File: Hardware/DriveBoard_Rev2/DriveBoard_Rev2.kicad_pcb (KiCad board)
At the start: 2 copper layers, 152.4 x 101.6 mm, 139 parts, among them J1 RJ45_LED_Shielded, Q1 Q_NMOS_DGS, Q2 Q_NMOS_DGS, Q3 Q_NMOS_DGS, Q4 Q_NMOS_DGS, Q5 Q_NMOS_DGS, Q6 Q_NMOS_DGS, Q7 Q_NMOS_DGS, Q8 Q_NMOS_DGS, Q9 Q_NMOS_DGS, SW1 SW_Push, SW10 SW_Push, SW11 SW_Push, SW12 SW_Push, SW13 SW_Push, SW14 SW_Push, SW15 SW_Push, SW16 SW_SPDT, SW2 SW_Push, SW3 SW_Push, SW4 SW_Push, SW5 SW_Push, SW6 SW_Push, SW7 SW_Push, SW8 SW_Push, SW9 SW_Push, U1 Teensy4.1_DEV-16771, U2 TSR_1-2450, U3 OKI, U4 74HC148, U5 74HC148, U6 74HC00, U7 TSR_1-2450

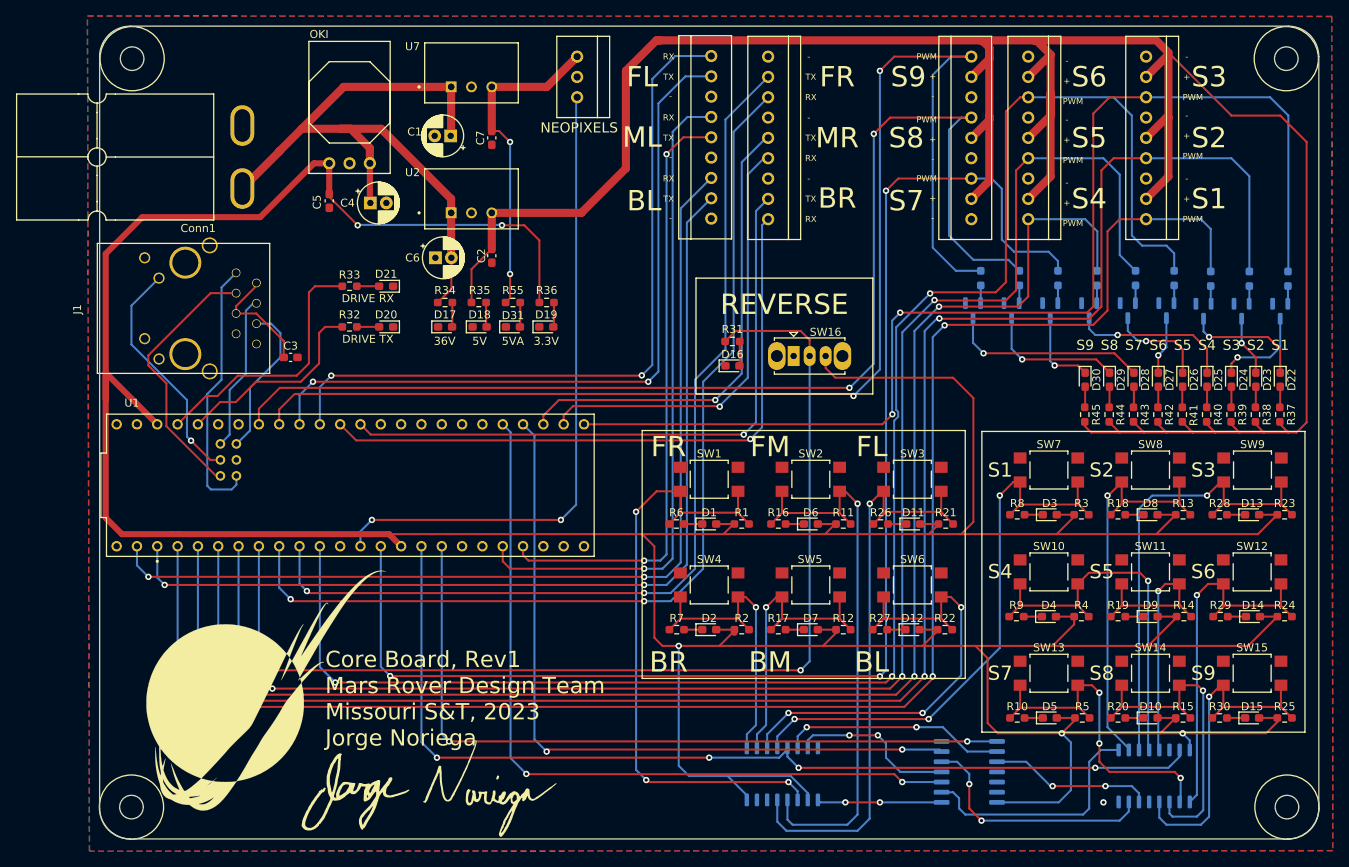
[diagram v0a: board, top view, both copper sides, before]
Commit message: Final Core Board
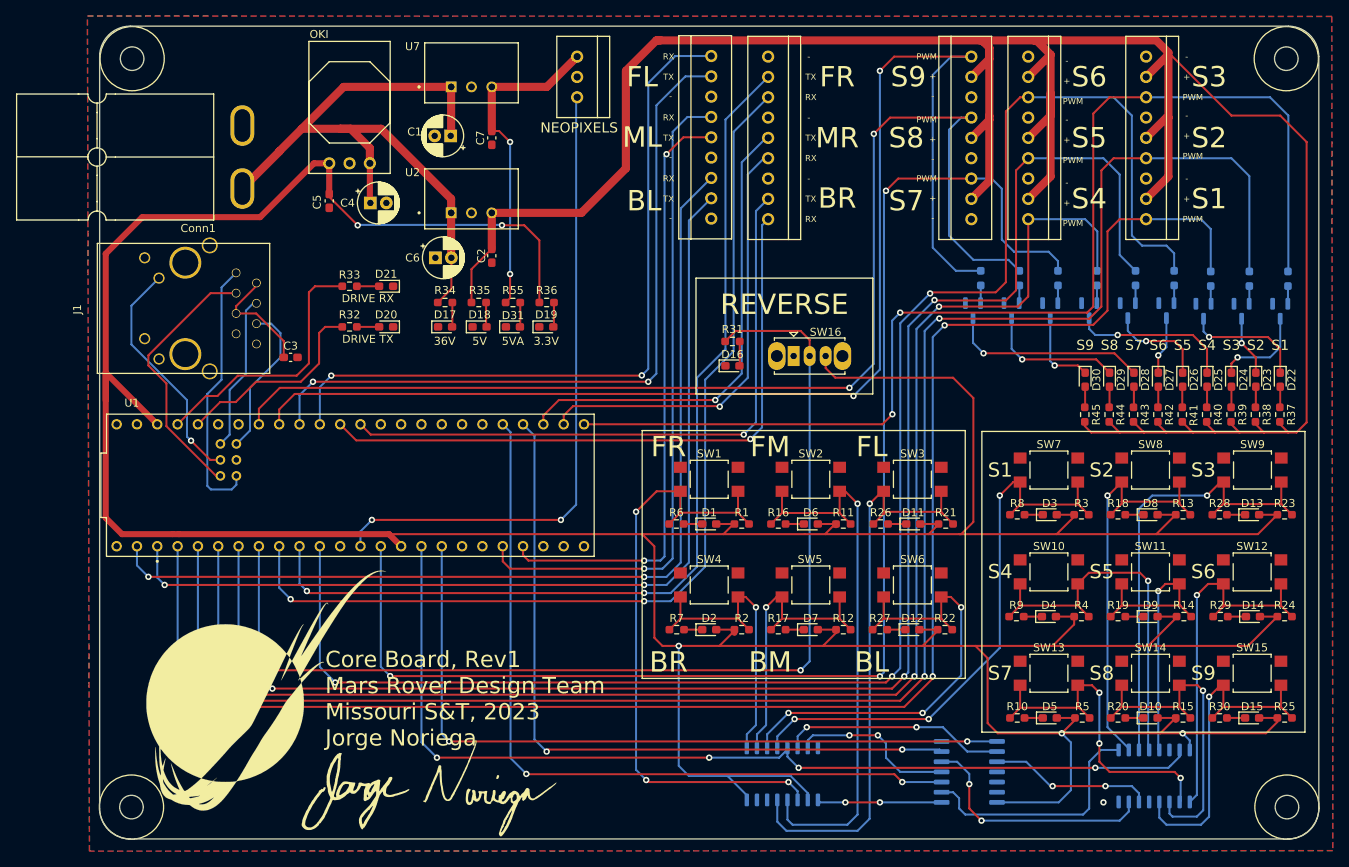
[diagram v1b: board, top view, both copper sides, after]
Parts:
- moved G*** 0.06 mm to (72.4, 134.1)
